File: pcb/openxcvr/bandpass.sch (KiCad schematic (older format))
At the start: 39 parts, among them U6 74LS251, U7 74LS251

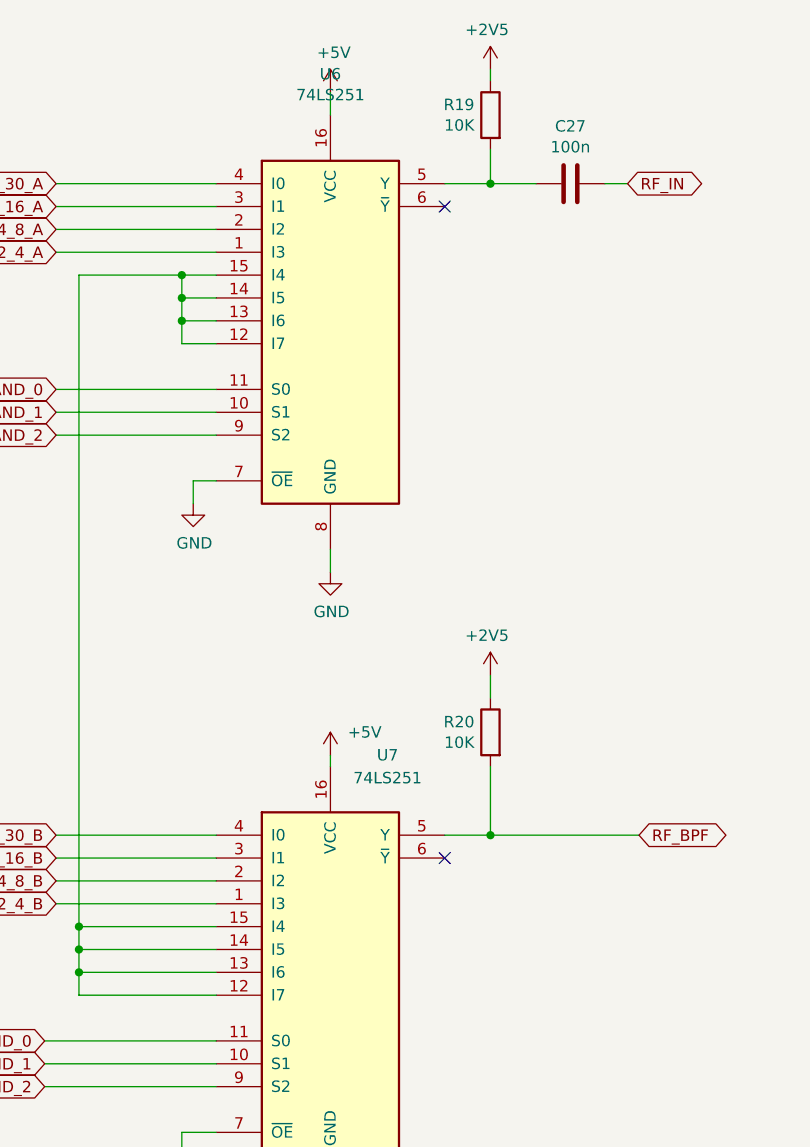
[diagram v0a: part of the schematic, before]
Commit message: Review and update schematic
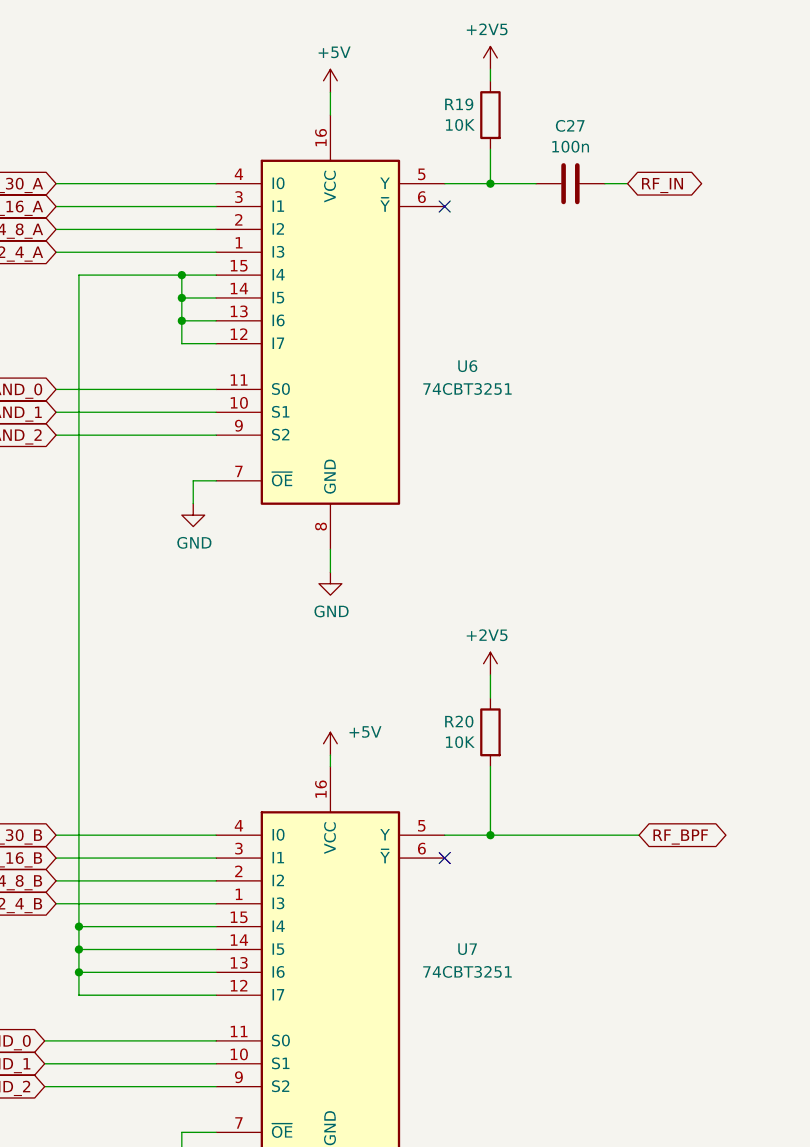
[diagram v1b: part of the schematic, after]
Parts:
- U6, U7: value 74LS251 -> 74CBT3251
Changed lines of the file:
@@
 U 1 1 5E6F0B24
 P 3200 2400
-F 0 "U6" H 3200 3479 50  0000 C CNN
-F 1 "74LS251" H 3200 3388 50  0000 C CNN
+F 0 "U6" H 3800 2200 50  0000 C CNN
+F 1 "74CBT3251" H 3800 2100 50  0000 C CNN
 F 2 "Package_SO:SOIC-16_3.9x9.9mm_P1.27mm" H 3200 2400 50  0001 C CNN
 F 3 "http://www.ti.com/lit/gpn/sn74LS251" H 3200 2400 50  0001 C CNN
@@
 U 1 1 5E723939
 P 3200 5250
-F 0 "U7" H 3450 6200 50  0000 C CNN
-F 1 "74LS251" H 3450 6100 50  0000 C CNN
+F 0 "U7" H 3800 5350 50  0000 C CNN
+F 1 "74CBT3251" H 3800 5250 50  0000 C CNN
 F 2 "Package_SO:SOIC-16_3.9x9.9mm_P1.27mm" H 3200 5250 50  0001 C CNN
 F 3 "http://www.ti.com/lit/gpn/sn74LS251" H 3200 5250 50  0001 C CNN
